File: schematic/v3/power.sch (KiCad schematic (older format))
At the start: 17 parts, among them IC1 MCP73831/2, J13 LIPO_BAT, SW1 RS stock no. 448-0747, U1 TLV71333PDBV, U3 TLV71333PDBV

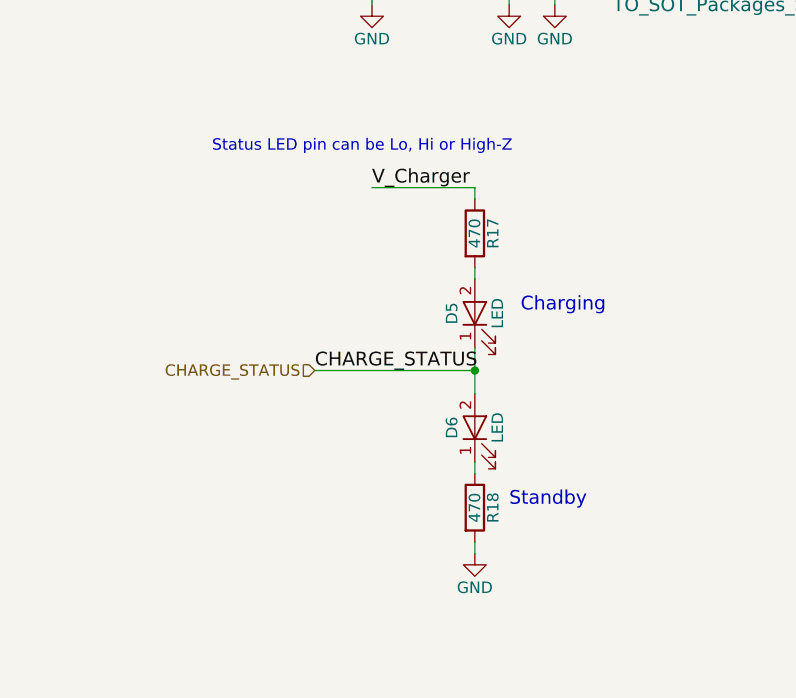
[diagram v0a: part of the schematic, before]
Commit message: More layout work
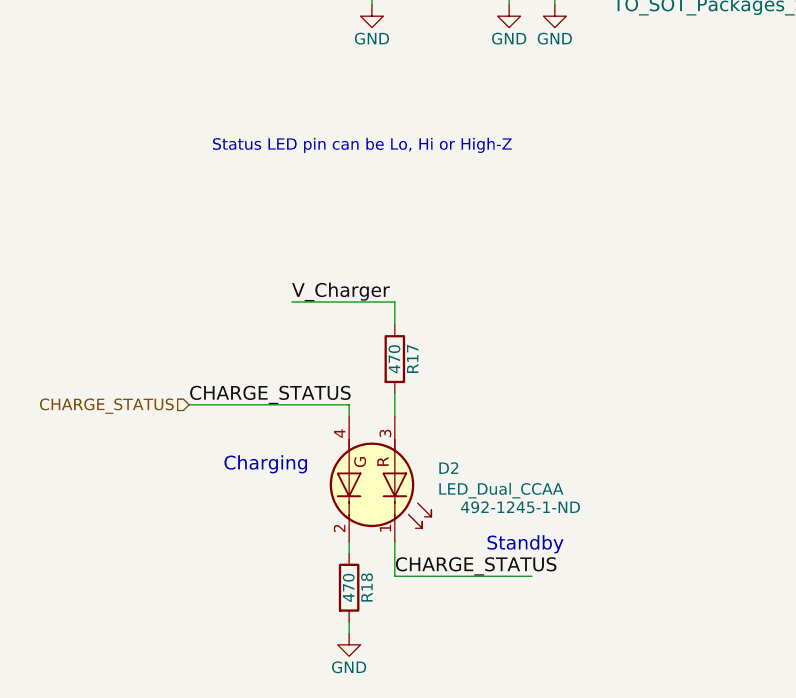
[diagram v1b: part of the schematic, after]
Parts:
- removed D5, D6: LED, LEDs:LED_0805_HandSoldering, symbol gps_node-rescue:LED
- added D2: LED_Dual_CCAA, dual_led:LED_DUAL_1206, symbol led_dual_ccaa:LED_Dual_CCAA
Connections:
- wire segments 67 -> 68
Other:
- moved on the sheet: R17, R18
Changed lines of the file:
@@
 Text Label 2850 3750 0    60   ~ 0
 CHARGE_STATUS
-Text Label 2400 5850 0    60   ~ 0
+Text Label 2750 6750 0    60   ~ 0
 CHARGE_STATUS
-$Comp
-L gps_node-rescue:LED D5
-U 1 1 5BFDCD72
-P 3100 5600
-F 0 "D5" H 3100 5700 50  0000 C CNN
-F 1 "LED" H 3100 5500 50  0000 C CNN
-F 2 "LEDs:LED_0805_HandSoldering" H 3100 5600 50  0001 C CNN
-F 3 "" H 3100 5600 50  0001 C CNN
-	1    3100 5600
-	0    -1   -1   0
-$EndComp
-$Comp
-L gps_node-rescue:LED D6
-U 1 1 5BFDCD79
-P 3100 6100
-F 0 "D6" H 3100 6200 50  0000 C CNN
-F 1 "LED" H 3100 6000 50  0000 C CNN
-F 2 "LEDs:LED_0805_HandSoldering" H 3100 6100 50  0001 C CNN
-F 3 "" H 3100 6100 50  0001 C CNN
-	1    3100 6100
-	0    -1   -1   0
-$EndComp
 $Comp
 L gps_node-rescue:R R18
 U 1 1 5BFDCD80
-P 3100 6450
-F 0 "R18" V 3180 6450 50  0000 C CNN
-F 1 "470" V 3100 6450 50  0000 C CNN
-F 2 "Resistors_SMD:R_0805" V 3030 6450 50  0001 C CNN
-F 3 "" H 3100 6450 50  0001 C CNN
-	1    3100 6450
+P 2550 6800
+F 0 "R18" V 2630 6800 50  0000 C CNN
+F 1 "470" V 2550 6800 50  0000 C CNN
+F 2 "Resistors_SMD:R_0805" V 2480 6800 50  0001 C CNN
+F 3 "" H 2550 6800 50  0001 C CNN
+	1    2550 6800
 	1    0    0    -1
 $EndComp
@@
 L gps_node-rescue:R R17
 U 1 1 5BFDCD87
-P 3100 5250
-F 0 "R17" V 3180 5250 50  0000 C CNN
-F 1 "470" V 3100 5250 50  0000 C CNN
-F 2 "Resistors_SMD:R_0805" V 3030 5250 50  0001 C CNN
-F 3 "" H 3100 5250 50  0001 C CNN
-	1    3100 5250
+P 2750 5800
+F 0 "R17" V 2830 5800 50  0000 C CNN
+F 1 "470" V 2750 5800 50  0000 C CNN
+F 2 "Resistors_SMD:R_0805" V 2680 5800 50  0001 C CNN
+F 3 "" H 2750 5800 50  0001 C CNN
+	1    2750 5800
 	1    0    0    -1
 $EndComp
@@
 L gps_node-rescue:GND-power #PWR0112
 U 1 1 5BFDCD8E
-P 3100 6650
-F 0 "#PWR0112" H 3100 6400 50  0001 C CNN
-F 1 "GND" H 3100 6500 50  0000 C CNN
-F 2 "" H 3100 6650 50  0001 C CNN
-F 3 "" H 3100 6650 50  0001 C CNN
-	1    3100 6650
+P 2550 7000
+F 0 "#PWR0112" H 2550 6750 50  0001 C CNN
+F 1 "GND" H 2550 6850 50  0000 C CNN
+F 2 "" H 2550 7000 50  0001 C CNN
+F 3 "" H 2550 7000 50  0001 C CNN
+	1    2550 7000
 	1    0    0    -1
 $EndComp
 Text Label 2800 3650 0    60   ~ 0
 V_Charger
-Text Label 2650 5050 0    60   ~ 0
+Text Label 2300 5550 0    60   ~ 0
 V_Charger
-Text Notes 3300 5600 0    60   ~ 0
+Text Notes 2000 6300 0    60   ~ 0
 Charging
-Text Notes 3250 6450 0    60   ~ 0
+Text Notes 3150 6650 0    60   ~ 0
 Standby
 $Comp
@@
 	2850 3750 3450 3750
 Wire Wire Line
-	2400 5850 3100 5850
-Wire Wire Line
-	3100 6600 3100 6650
-Wire Wire Line
-	3100 6300 3100 6250
-Wire Wire Line
-	3100 5750 3100 5850
-Connection ~ 3100 5850
-Wire Wire Line
-	3100 5450 3100 5400
-Wire Wire Line
-	2650 5050 3100 5050
-Wire Wire Line
-	3100 5050 3100 5100
+	2300 5550 2750 5550
 Wire Wire Line
 	7100 1950 7100 1850
@@
 Wire Wire Line
 	8450 3800 8050 3800
-Wire Wire Line
-	3100 5850 3100 5950
 Wire Wire Line
 	7100 1850 7750 1850
@@
 Text Notes 6750 4950 0    101  ~ 0
 Global power labels
-Text HLabel 2400 5850 0    50   Input ~ 0
+Text HLabel 1850 6000 0    50   Input ~ 0
 CHARGE_STATUS
 $Comp
@@
 	1    0    0    -1
 $EndComp
+Text Label 1850 6000 0    60   ~ 0
+CHARGE_STATUS
+Wire Wire Line
+	1850 6000 2550 6000
+Wire Wire Line
+	2750 5550 2750 5650
+Wire Wire Line
+	2550 6650 2550 6600
+Wire Wire Line
+	2550 7000 2550 6950
+Wire Wire Line
+	2750 6750 3350 6750
+$Comp
+L led_dual_ccaa:LED_Dual_CCAA D2
+U 1 1 5BE716E8
+P 2650 6350
+F 0 "D2" V 2579 6638 50  0000 L CNN
+F 1 "LED_Dual_CCAA" V 2670 6638 50  0000 L CNN
+F 2 "dual_led:LED_DUAL_1206" H 2680 6350 50  0001 C CNN
+F 3 "~" H 2680 6350 50  0001 C CNN
+F 4 "492-1245-1-ND" V 2750 7000 50  0000 C CNN "Digikey"
+	1    2650 6350
+	0    1    1    0
+$EndComp
+Wire Wire Line
+	2750 6600 2750 6750
+Wire Wire Line
+	2750 5950 2750 6050
+Wire Wire Line
+	2550 6000 2550 6050
 $EndSCHEMATC
